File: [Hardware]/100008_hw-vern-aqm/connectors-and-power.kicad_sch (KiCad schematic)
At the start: 16 parts

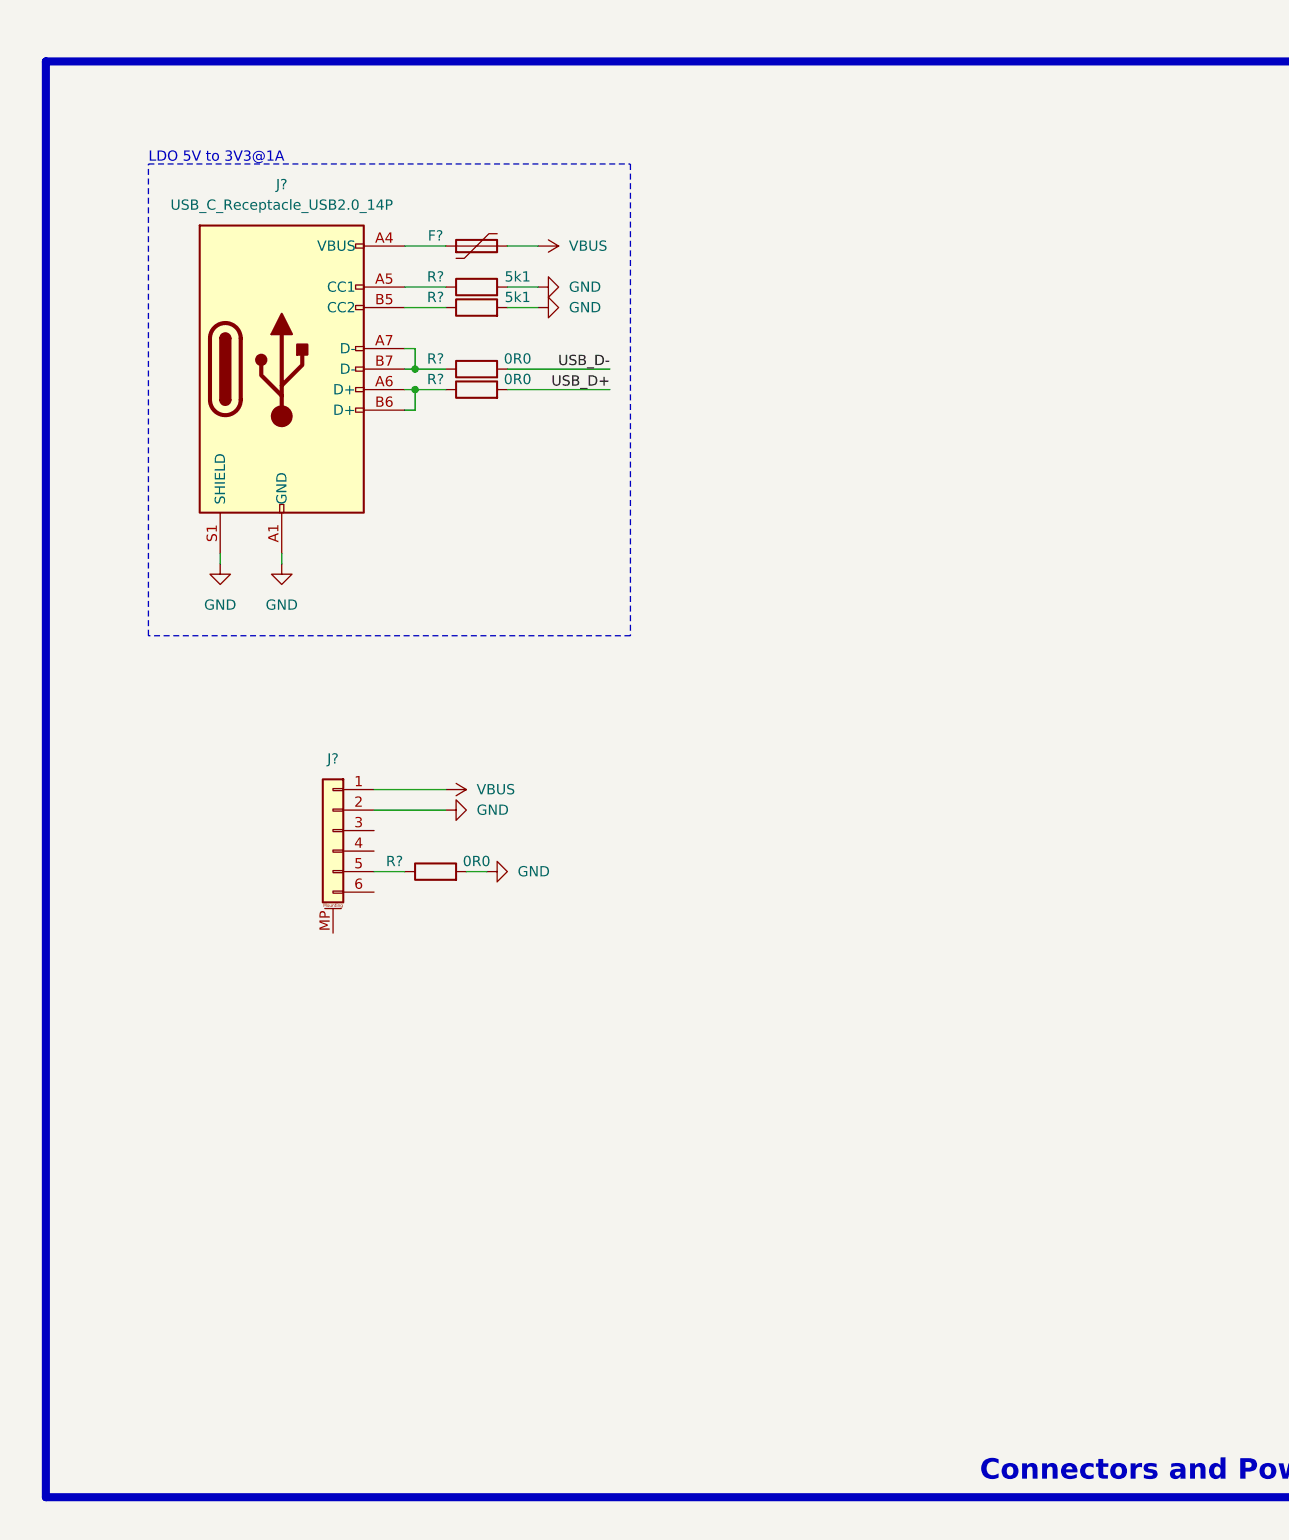
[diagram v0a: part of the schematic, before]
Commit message: end of day work
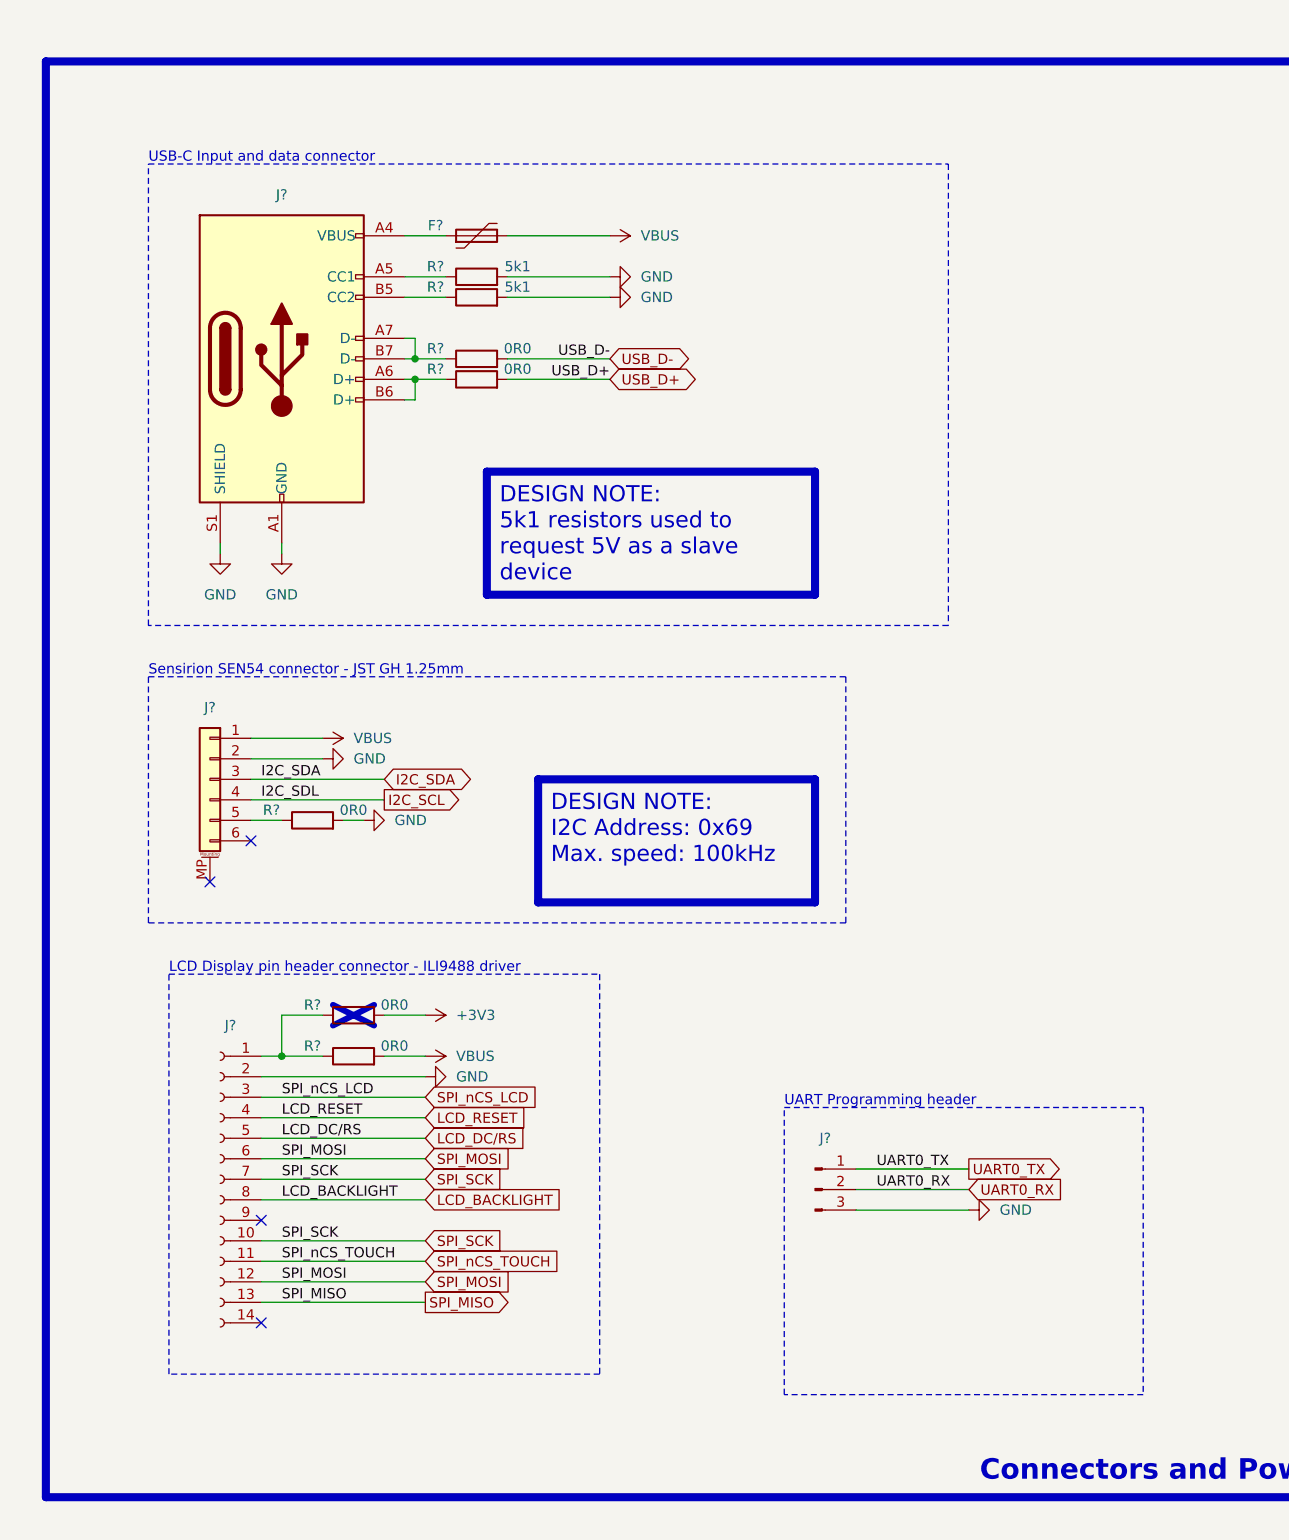
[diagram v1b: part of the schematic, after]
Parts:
- added J?: Conn_01x03_Pin, symbol Connector:Conn_01x03_Pin
- added J?: Conn_01x14_Socket, symbol Connector:Conn_01x14_Socket
- added R? (x2): 0R0, Resistor_SMD:R_0603_1608Metric, symbol Device:R
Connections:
- net +3V3: now also R?.2
- net GND: now also J?.2 (Pin_2), J?.3 (Pin_3)
- net VBUS: now also R?.2
- net I2C_SDA: now reaches J?.3 (Pin_3)
- net I2C_SCL: now reaches J?.4 (Pin_4)
- new net: J?.1 (Pin_1), R?.1, R?.1
- new net LCD_BACKLIGHT: J?.8 (Pin_8)
- new net LCD_DC/RS: J?.5 (Pin_5)
- new net LCD_RESET: J?.4 (Pin_4)
- new net SPI_MISO: J?.13 (Pin_13)
- new net SPI_MOSI: J?.12 (Pin_12), J?.6 (Pin_6)
- new net SPI_SCK: J?.10 (Pin_10), J?.7 (Pin_7)
- new net SPI_nCS_LCD: J?.3 (Pin_3)
- new net SPI_nCS_TOUCH: J?.11 (Pin_11)
- new net UART0_RX: J?.2 (Pin_2)
- new net UART0_TX: J?.1 (Pin_1)
- no-connect marks 0 -> 4
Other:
- note added: "LCD Display pin header connector - ILI9488 driver"
- note added: "Sensirion SEN54 connector - JST GH 1.25mm"
- note added: "UART Programming header"
- note added: "USB-C Input and data connector"
- moved on the sheet: F?, J?, R?
